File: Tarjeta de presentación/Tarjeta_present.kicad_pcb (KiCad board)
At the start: 2 copper layers, 49.9 x 17.3 mm, 11 parts, among them J1 Conn_01x01_Female, J2 USB_A, SW1 Reset, SW2 Boot, U1 CH552G

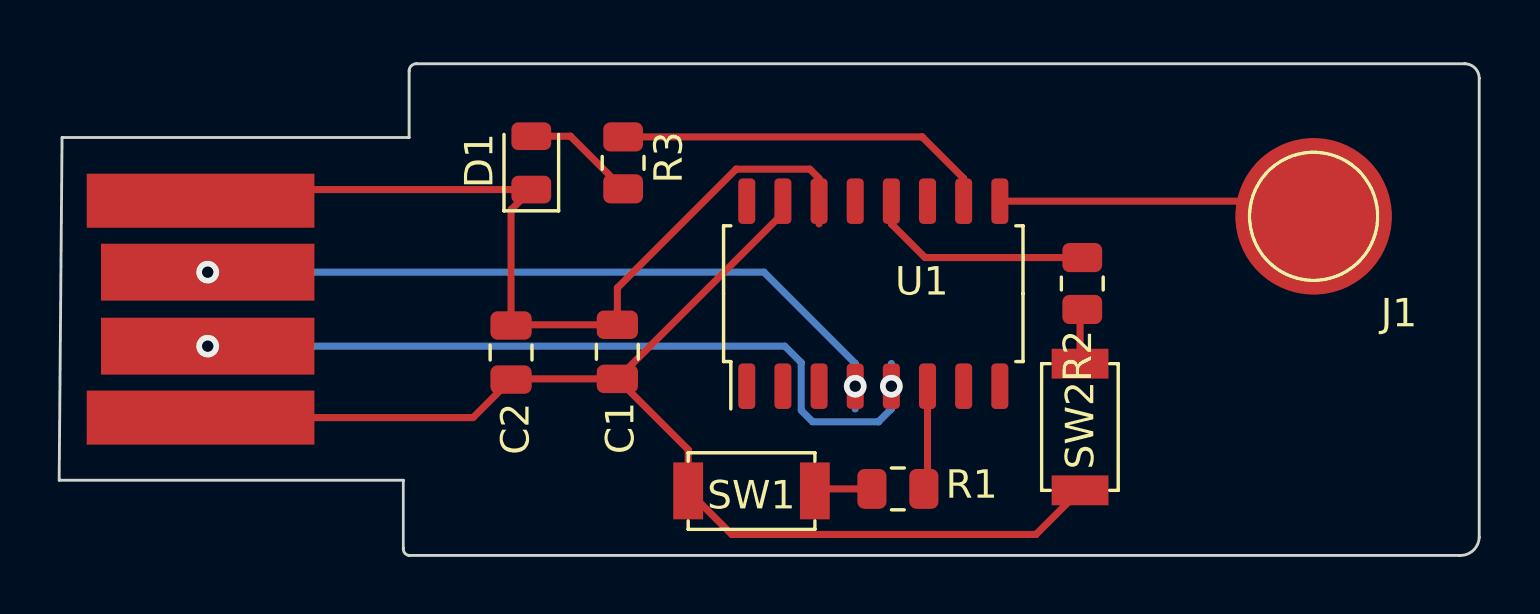
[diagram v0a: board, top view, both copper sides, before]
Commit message: Add ground template
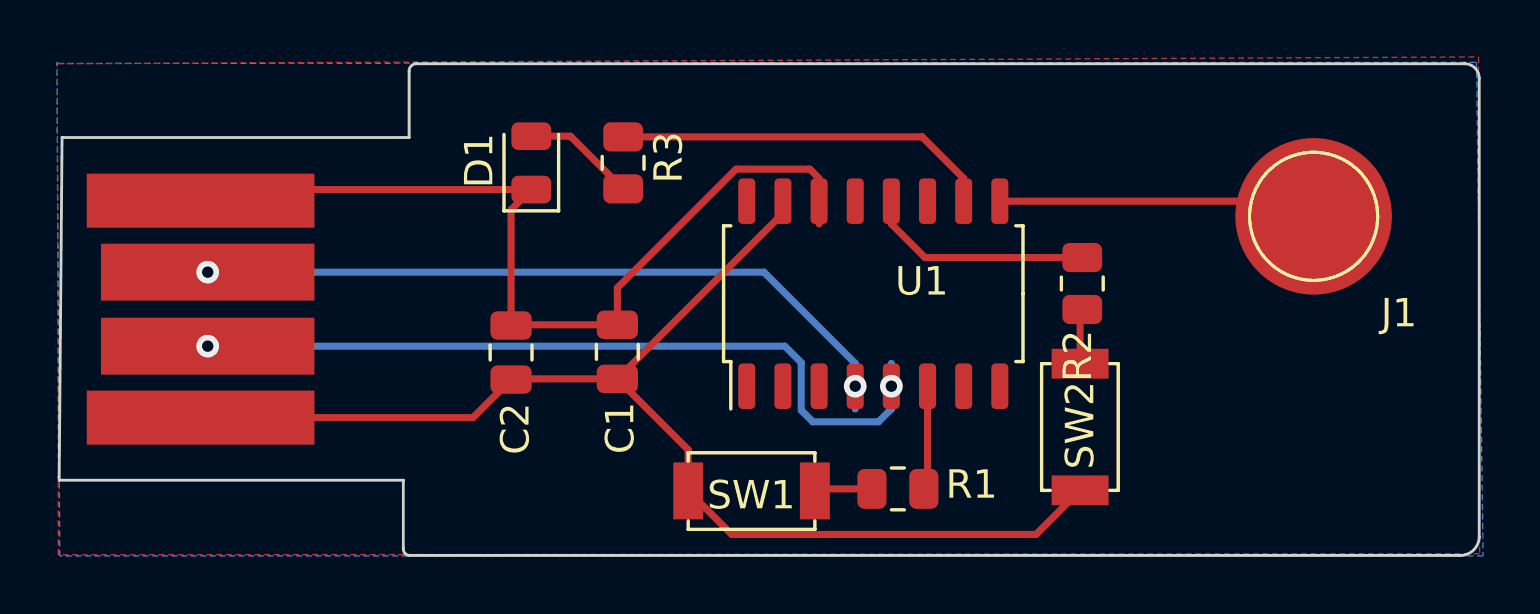
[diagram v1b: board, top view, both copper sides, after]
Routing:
- added copper zone on B.Cu, net (none)
- added copper zone on F.Cu, net GND
